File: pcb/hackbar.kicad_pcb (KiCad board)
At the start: 2 copper layers, 159 x 25 mm, 32 parts, among them SW1 SW_Push, SW2 SW_Push, SW3 SW_Push, SW4 SW_Push, SW5 SW_Push, SW6 SW_Push, SW7 SW_Push, U1 XIAO-RP2040-SMD

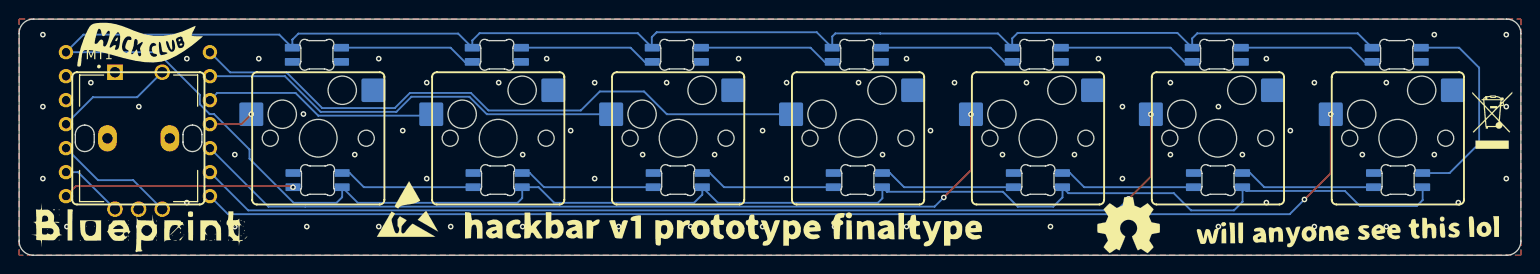
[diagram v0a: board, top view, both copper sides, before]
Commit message: add cad, images, readme, bom
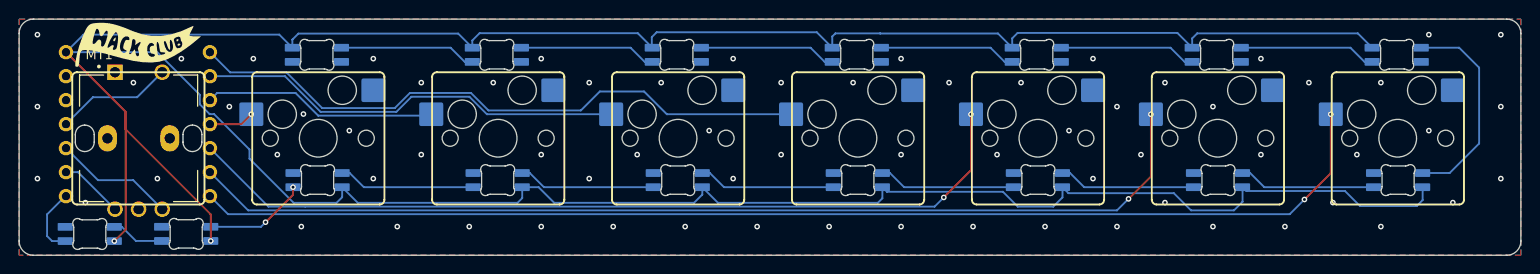
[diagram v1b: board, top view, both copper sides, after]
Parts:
- removed the G*** at (156.8, 69.4)
- removed the G*** at (156.3, 69.4)
- removed the REF** at (194.5, 78.8)
- removed the REF** at (118.1, 77.1)
- removed the REF** at (233.0, 67.7)
- removed the REF** at (232.2, 74.7)
- added D15: SK6812, 2_udu_lib:SK6812MINI-E_fixed, F.Cu at (84.5, 79.8)
- added D16: SK6812, 2_udu_lib:SK6812MINI-E_fixed, F.Cu at (94.7, 79.8)
- added G***: LOGO, 1_udu_lib:hackclub, F.Cu at (89.4, 60.0)
- added G***: LOGO, 1_udu_lib:hackbar_back2, B.Cu at (182.1, 79.7)
- added G***: LOGO, 1_udu_lib:blueprint, B.Cu at (201.8, 78.7)
- added G***: LOGO, 1_udu_lib:hackclub, B.Cu at (103.8, 79.4)
- added REF**: OSHW-Logo2_7.3x6mm_SilkScreen, Symbol:OSHW-Logo2_7.3x6mm_SilkScreen, B.Cu at (232.6, 75.5)
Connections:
- D1 pad 2: IO1 -> Net-(D1-DIN)
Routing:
- net +5V: track 317.2 -> 357.7 mm, vias 0 -> 2
- net IO1: track 24.5 -> 7.24 mm, vias 1 -> 0
- net Net-(D1-DIN): track 0.00 -> 10.9 mm, vias 0 -> 2
- net Net-(D15-DOUT): track 0.00 -> 5.63 mm
- net GND: vias 73 -> 69
